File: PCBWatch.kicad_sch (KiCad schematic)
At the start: 39 parts, among them J1 Conn_01x07_Pin, J2 Touch Electrode, J3 Conn_A_left, J4 Conn_B_left, J5 Conn_A_right, J6 Conn_B_right, U1 STM32L010C6Tx, U2 MCP23017_SS, U3 AT42QT1010-TSHR, Y1 32.768KHZ

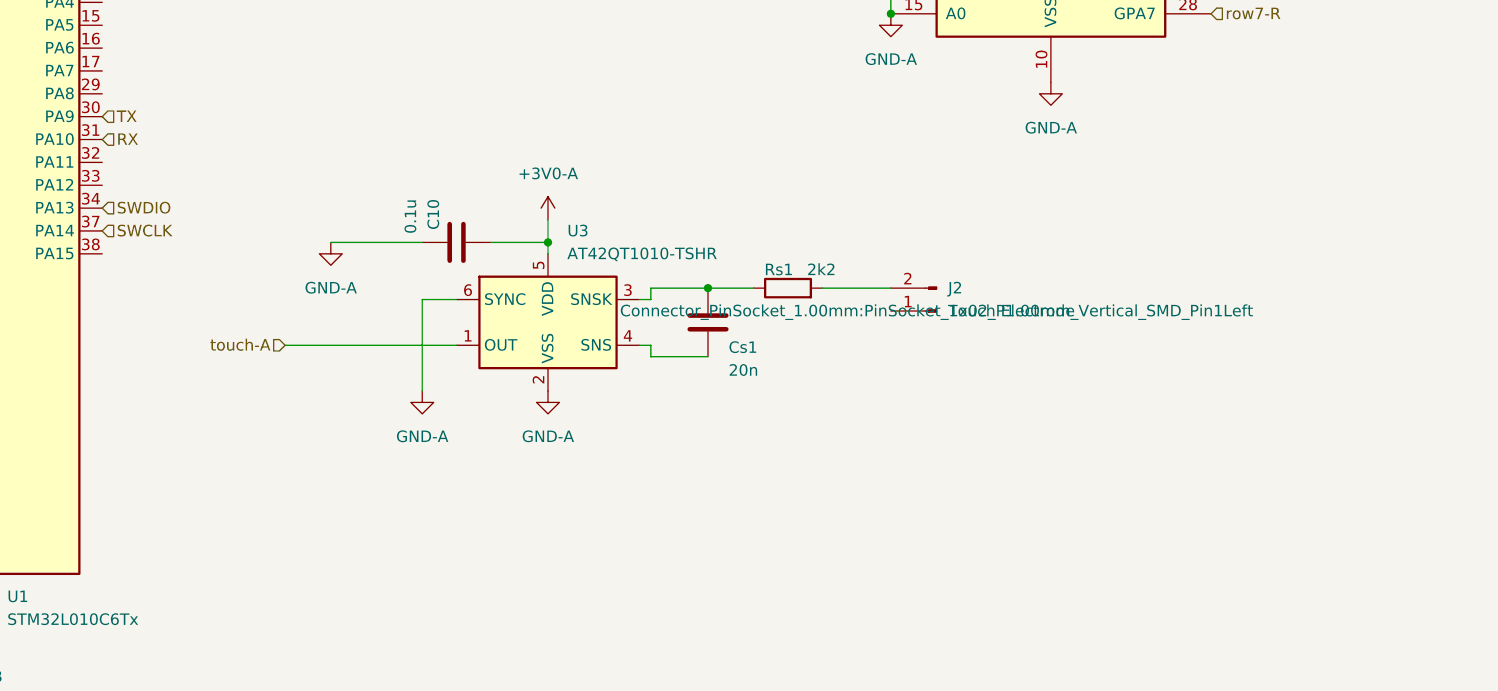
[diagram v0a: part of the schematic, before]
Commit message: Push old changes of version 3
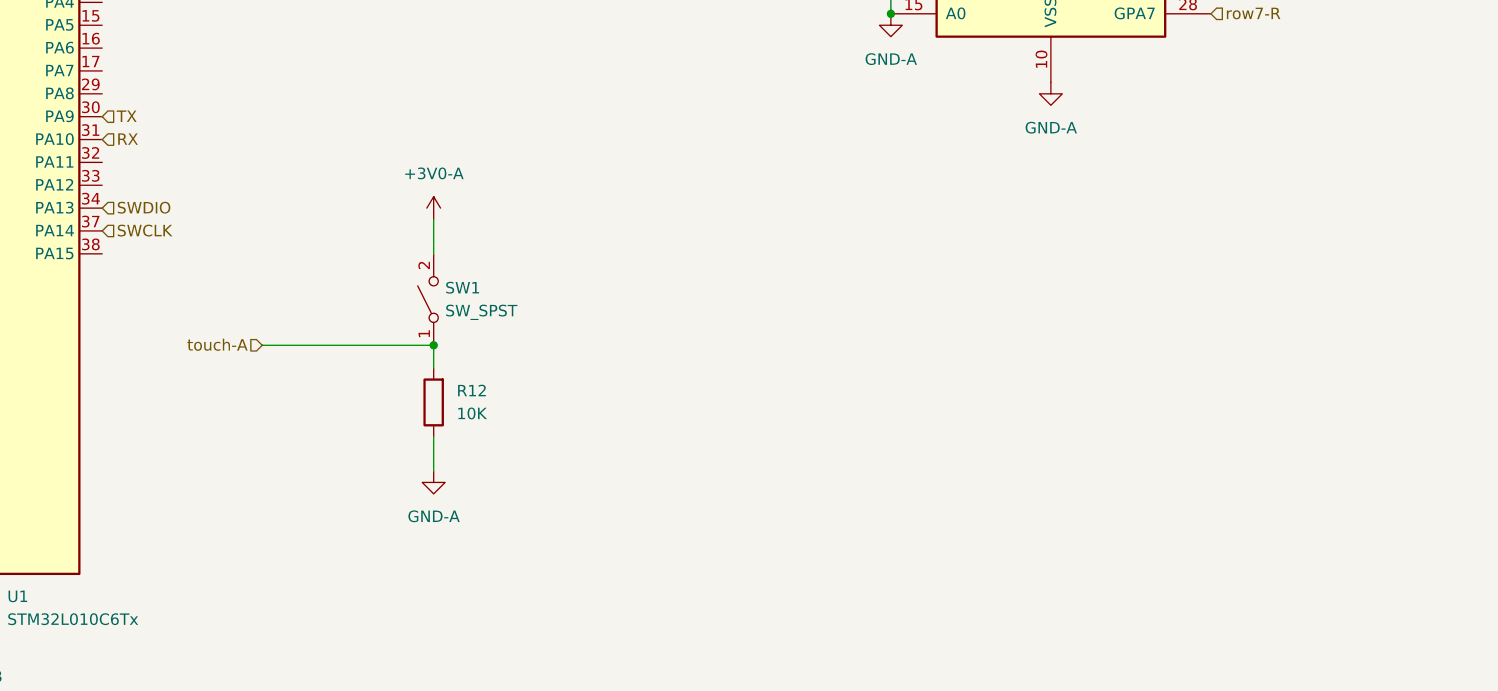
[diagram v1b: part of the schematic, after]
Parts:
- removed C10: 0.1u, Capacitor_SMD:C_0805_2012Metric, symbol Device:C
- removed Cs1: 20n, Capacitor_SMD:C_0805_2012Metric, symbol Device:C
- removed J2: Touch Electrode, Connector_PinSocket_1.00mm:PinSocket_1x02_P1.00mm_Vertical_SMD_Pin1Left, symbol Connector:Conn_01x02_Pin
- removed Rs1: 2k2, Resistor_SMD:R_0805_2012Metric, symbol Device:R
- removed U3: AT42QT1010-TSHR, Package_TO_SOT_SMD:SOT-23-6, symbol Sensor_Touch:AT42QT1010-TSHR
- added R12: 10K, Resistor_SMD:R_0805_2012Metric, symbol Device:R
- added SW1: SW_SPST, my_footprints:SKQYAAE010 Switch, symbol Switch:SW_SPST
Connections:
- net +3V0-A: now also SW1.2 (B)
- net GND-A: now also R12.1
- net touch-A: now also R12.2, SW1.1 (A)
